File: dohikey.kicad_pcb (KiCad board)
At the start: 2 copper layers, 61.5 x 53.5 mm, 11 parts, among them J1 Conn_01x04_Pin, J2 DHT11, J3 Motor, J4 Barrel_Jack_Switch_Pin3Ring, Q1 PN2222A

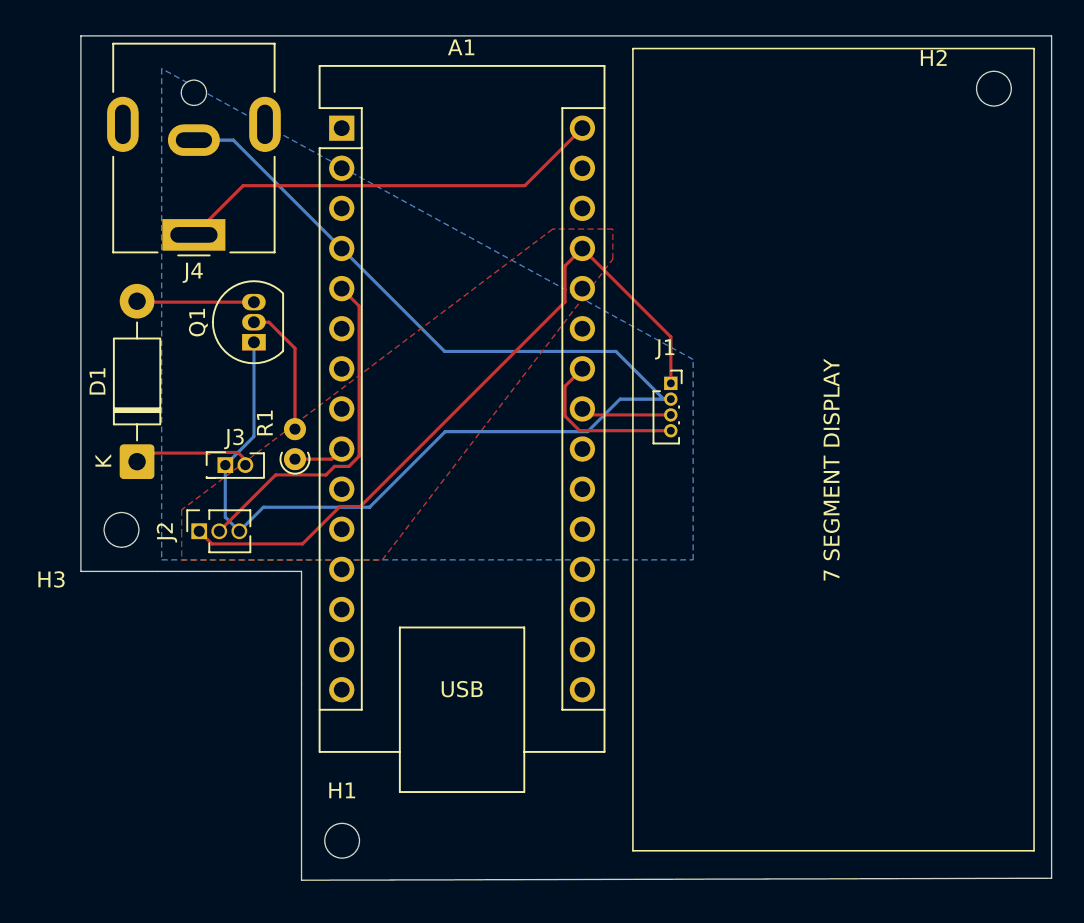
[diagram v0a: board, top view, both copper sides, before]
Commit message: Add files via upload
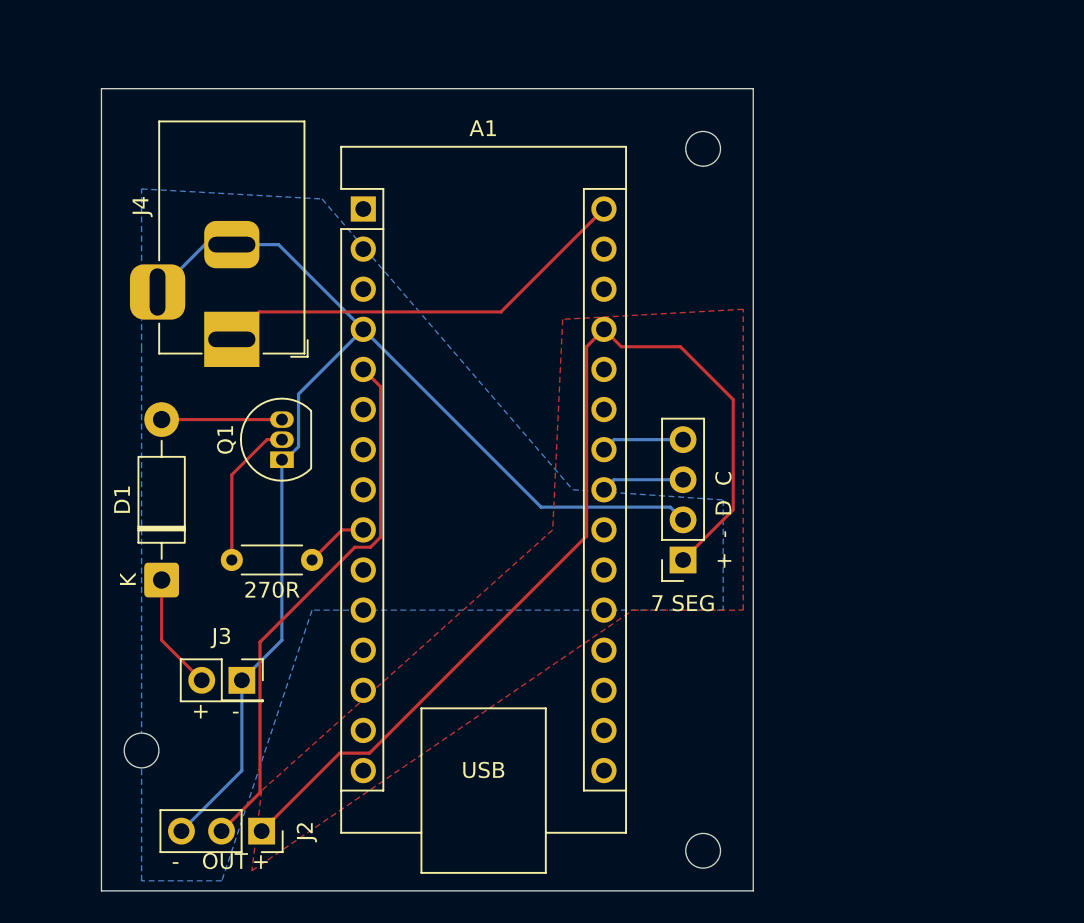
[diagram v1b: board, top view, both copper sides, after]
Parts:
- removed J1: Conn_01x04_Pin, Connector_PinSocket_1.00mm:PinSocket_1x04_P1.00mm_Vertical
- removed R1: 270, Resistor_THT:R_Axial_DIN0204_L3.6mm_D1.6mm_P1.90mm_Vertical
- added 270R: 270, Resistor_THT:R_Axial_DIN0204_L3.6mm_D1.6mm_P5.08mm_Horizontal, F.Cu at (55.9, 57.8)
- added 7 SEG: Conn_01x04_Pin, Connector_PinSocket_2.54mm:PinSocket_1x04_P2.54mm_Vertical, F.Cu at (79.4, 57.8)
- J2: footprint Connector_PinSocket_1.27mm:PinSocket_1x03_P1.27mm_Vertical -> Connector_PinSocket_2.54mm:PinSocket_1x03_P2.54mm_Vertical
- J3: footprint Connector_PinHeader_1.27mm:PinHeader_2x01_P1.27mm_Vertical -> Connector_PinSocket_2.54mm:PinSocket_2x01_P2.54mm_Vertical
- J4: footprint Connector_BarrelJack:BarrelJack_CUI_PJ-063AH_Horizontal -> Connector_BarrelJack:BarrelJack_Horizontal
- moved H1 22.9 mm to (80.6, 76.2)
- moved J2 19.4 mm to (52.7, 75.0), turned to -90 degrees
- moved H2 18.8 mm to (80.6, 31.8)
- moved H3 14.0 mm to (45.1, 69.8)
- moved J3 13.7 mm to (51.4, 65.4)
- moved D1 7.65 mm to (46.4, 59.1)
- moved Q1 7.64 mm to (54.0, 51.4)
- moved J4 7.04 mm to (50.8, 43.8), turned to -90 degrees
- moved A1 5.30 mm to (59.1, 35.6)
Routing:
- net +5V: track 44.5 -> 63.4 mm
- net Net-(A1-D2): track 21.9 -> 34.4 mm
- net Net-(A1-A5): track 10.5 -> 5.69 mm
- net GND: track 80.9 -> 78.4 mm
- net Net-(Q1-B): track 8.40 -> 9.49 mm
- net Net-(A1-D6): track 3.23 -> 4.03 mm
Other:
- board size 61.5 x 53.5 mm -> 41.3 x 50.8 mm
- board text added: "+"
- board text added: "+ - D C"
- board text added: "-"
- board text added: "OUT"
- board text added: "Temp & Humidity Sensor and Air Circulator Rev. 2 Jaxon Borges (March 18 2026)"
- board text removed: "7 SEGMENT DISPLAY"
- board text removed: "Temp & Humidity Sensor and Air Circulator Rev. 1 Jaxon Borges (March 2026)"
